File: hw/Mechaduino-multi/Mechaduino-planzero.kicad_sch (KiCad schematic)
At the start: 29 parts, among them IC1 A4954ELPTR-T, J2 SPI, J3 SPI_PWR, J4 Conn_01x04, J5 Conn_01x02, U1 ATtiny24-20MU, U2 AS5047D, U3 TLV70033_SOT353

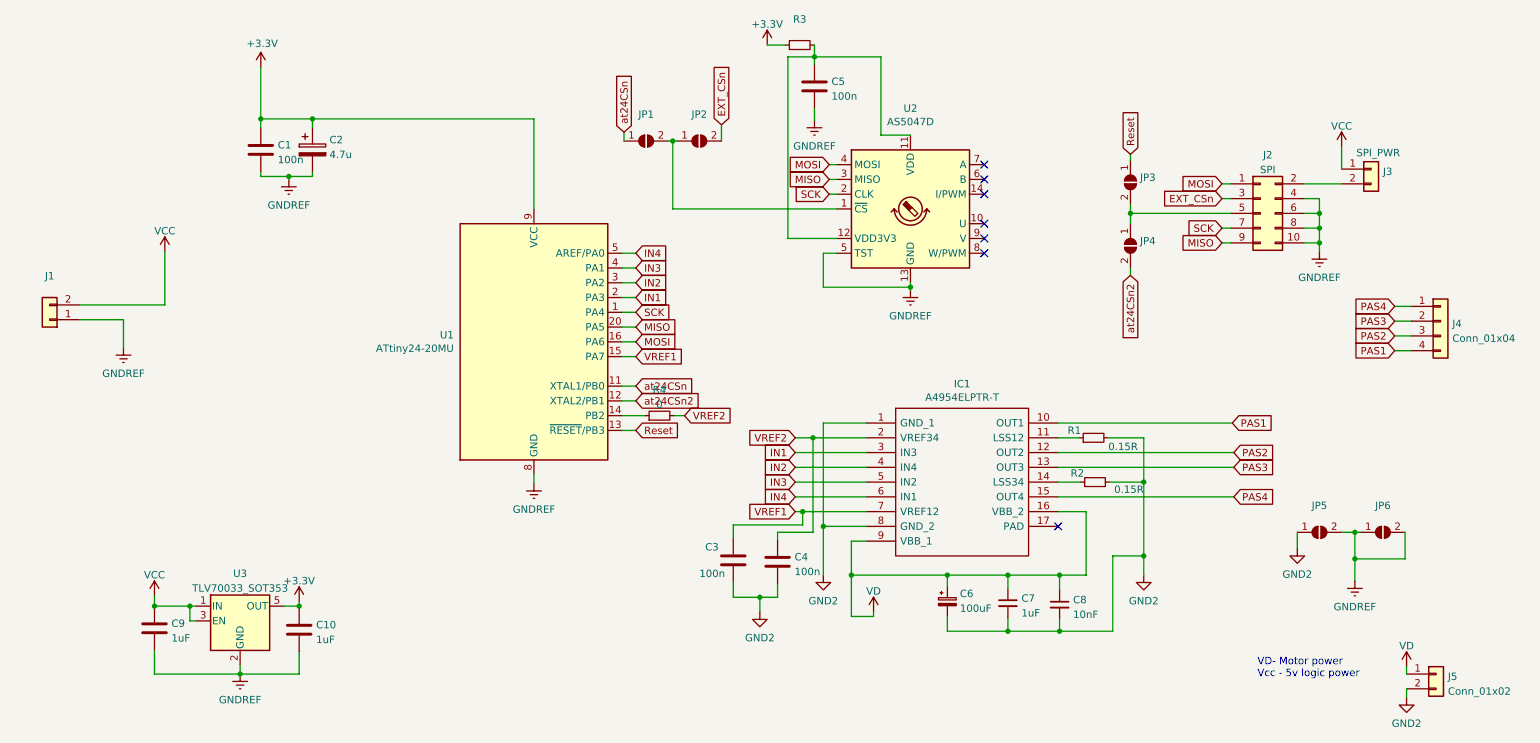
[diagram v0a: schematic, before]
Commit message: Add new updates to driver sch / layout
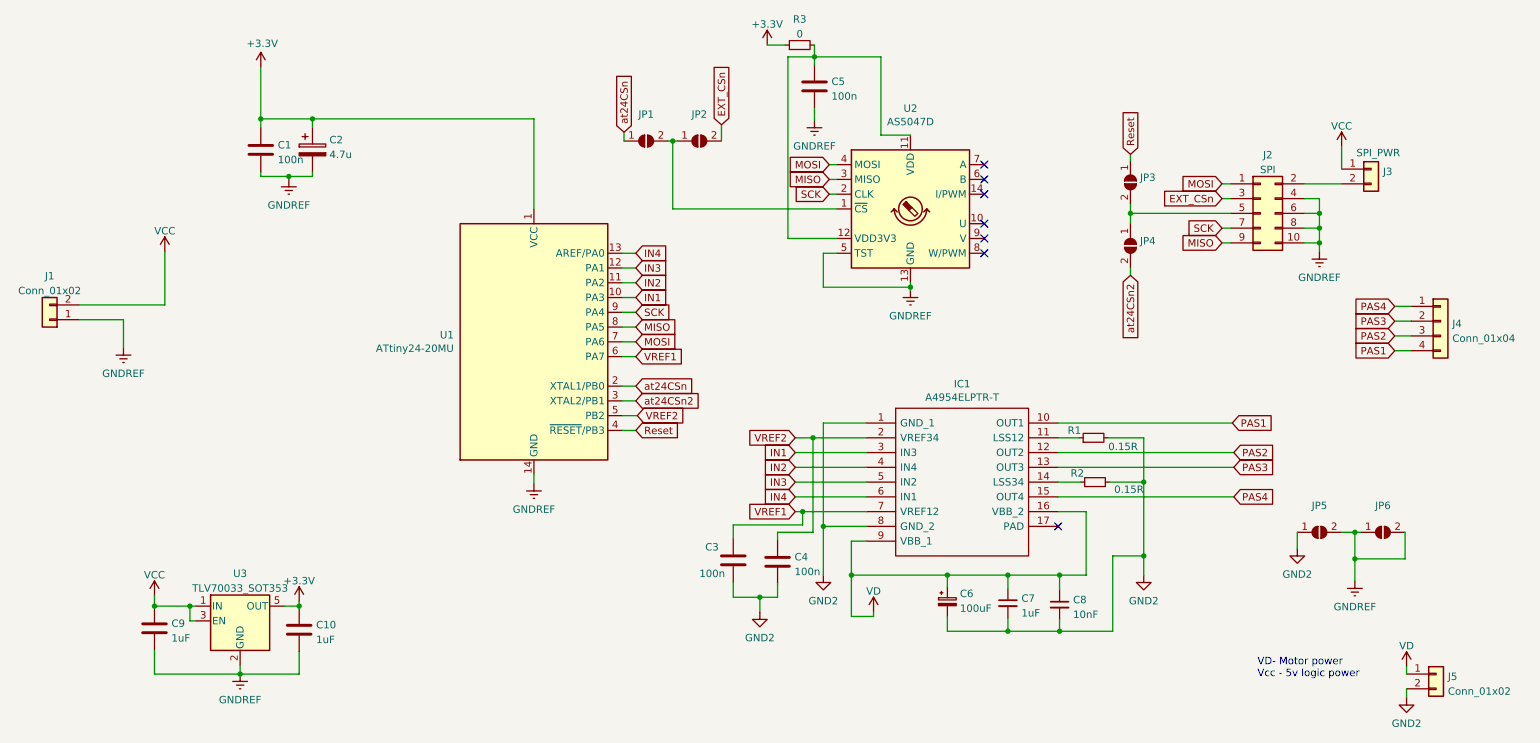
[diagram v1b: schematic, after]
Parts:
- removed R4: 0, Resistor_SMD:R_0805_2012Metric_Pad1.20x1.40mm_HandSolder, symbol Device:R_Small
- IC1: footprint (none) -> Package_SO:TSSOP-16-1EP_4.4x5mm_P0.65mm_EP3x3mm
- J1: value (none) -> Conn_01x02; footprint (none) -> Connector_PinSocket_2.54mm:PinSocket_1x02_P2.54mm_Horizontal
- J3: footprint (none) -> Connector_PinSocket_2.54mm:PinSocket_1x02_P2.54mm_Vertical
- R3: value (none) -> 0; footprint (none) -> Resistor_SMD:R_0805_2012Metric_Pad1.20x1.40mm_HandSolder
- U1: footprint Package_DFN_QFN:QFN-20-1EP_4x4mm_P0.5mm_EP2.6x2.6mm -> Package_SO:SOIC-14_3.9x8.7mm_P1.27mm; symbol Mechaduino-planzero-rescue:ATtiny24-20MU-MCU_Microchip_ATtiny -> MCU_Microchip_ATtiny:ATtiny24-20SSU
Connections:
- net +3V3: now also U1.1 (VCC); no longer U1.9 (VCC)
- net GNDREF: now also U1.14 (GND); no longer U1.21 (GND), U1.8 (GND)
- net IN1: now also U1.10 (PA3); no longer U1.2 (PA3)
- net IN2: now also U1.11 (PA2); no longer U1.3 (PA2)
- net IN3: now also U1.12 (PA1); no longer U1.4 (PA1)
- net IN4: now also U1.13 (AREF/PA0); no longer U1.5 (AREF/PA0)
- net MISO: now also U1.8 (PA5); no longer U1.20 (PA5)
- net MOSI: now also U1.7 (PA6); no longer U1.16 (PA6)
- net Reset: now also U1.4 (~{RESET}/PB3); no longer U1.13 (~{RESET}/PB3)
- net SCK: now also U1.9 (PA4); no longer U1.1 (PA4)
- net VREF1: now also U1.6 (PA7); no longer U1.15 (PA7)
- net VREF2: now also U1.5 (PB2)
- net at24CSn: now also U1.2 (XTAL1/PB0); no longer U1.11 (XTAL1/PB0)
- net at24CSn2: now also U1.3 (XTAL2/PB1); no longer U1.12 (XTAL2/PB1)
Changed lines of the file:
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@@
-    (stroke (width 0) (type default) (color 0 0 0 0))
-  )
-  (wire (pts (xy 137.16 81.28) (xy 138.938 81.28))
     (stroke (width 0) (type default) (color 0 0 0 0))
   )
@@
     (stroke (width 0) (type default) (color 0 0 0 0))
   )
-  (wire (pts (xy 128.27 81.28) (xy 132.08 81.28))
+  (wire (pts (xy 128.27 81.28) (xy 130.81 81.28))
     (stroke (width 0) (type default) (color 0 0 0 0))
   )
@@
     )
   )
-  (global_label "VREF2" (shape input) (at 138.938 81.28 0) (fields_autoplaced)
-    (effects (font (size 1.27 1.27)) (justify left))
-    (property "Intersheet References" "${INTERSHEET_REFS}" (id 0) (at 147.0679 81.2006 0)
+  (global_label "VREF2" (shape input) (at 130.81 81.28 0) (fields_autoplaced)
+    (effects (font (size 1.27 1.27)) (justify left))
+    (property "Intersheet References" "${INTERSHEET_REFS}" (id 0) (at 138.9399 81.2006 0)
       (effects (font (size 1.27 1.27)) (justify left) hide)
     )
@@
     (property "Reference" "IC1" (id 0) (at 186.69 75.819 0))
     (property "Value" "A4954ELPTR-T" (id 1) (at 186.69 78.1304 0))
-    (property "Footprint" "" (id 2) (at 199.39 80.01 0)
+    (property "Footprint" "Package_SO:TSSOP-16-1EP_4.4x5mm_P0.65mm_EP3x3mm" (id 2) (at 199.39 80.01 0)
       (effects (font (size 1.27 1.27)) (justify left) hide)
     )
@@
     (pin "9")
   )
-  (symbol (lib_id "Mechaduino-planzero-rescue:ATtiny24-20MU-MCU_Microchip_ATtiny") (at 113.03 68.58 0) (unit 1)
+  (symbol (lib_id "MCU_Microchip_ATtiny:ATtiny24-20SSU") (at 113.03 68.58 0) (unit 1)
     (in_bom yes) (on_board yes)
     (property "Reference" "U1" (id 0) (at 99.2378 67.4116 0)
@@
       (effects (font (size 1.27 1.27)) (justify right))
     )
-    (property "Footprint" "Package_DFN_QFN:QFN-20-1EP_4x4mm_P0.5mm_EP2.6x2.6mm" (id 2) (at 113.03 68.58 0)
+    (property "Footprint" "Package_SO:SOIC-14_3.9x8.7mm_P1.27mm" (id 2) (at 113.03 68.58 0)
       (effects (font (size 1.27 1.27) italic) hide)
     )
@@
     (pin "13")
     (pin "14")
-    (pin "15")
-    (pin "16")
-    (pin "17")
-    (pin "18")
-    (pin "19")
-    (pin "2")
-    (pin "20")
-    (pin "21")
+    (pin "2")
     (pin "3")
     (pin "4")
@@
     (in_bom yes) (on_board yes) (fields_autoplaced)
     (property "Reference" "R3" (id 0) (at 158.75 13.0896 90))
-    (property "Value" "" (id 1) (at 158.75 15.6265 90))
-    (property "Footprint" "" (id 2) (at 158.75 17.526 0)
+    (property "Value" "0" (id 1) (at 158.75 15.6265 90))
+    (property "Footprint" "Resistor_SMD:R_0805_2012Metric_Pad1.20x1.40mm_HandSolder" (id 2) (at 158.75 17.526 0)
       (effects (font (size 1.27 1.27)) hide)
     )
@@
       (effects (font (size 1.27 1.27)) (justify left))
     )
-    (property "Footprint" "" (id 2) (at 257.048 38.862 0)
+    (property "Footprint" "Connector_PinSocket_2.54mm:PinSocket_1x02_P2.54mm_Vertical" (id 2) (at 257.048 38.862 0)
       (effects (font (size 1.27 1.27)) hide)
     )
@@
     (pin "1")
   )
-  (symbol (lib_id "Device:R_Small") (at 134.62 81.28 90) (unit 1)
-    (in_bom yes) (on_board yes) (fields_autoplaced)
-    (property "Reference" "R4" (id 0) (at 134.62 76.8436 90))
-    (property "Value" "0" (id 1) (at 134.62 79.3805 90))
-    (property "Footprint" "Resistor_SMD:R_0805_2012Metric_Pad1.20x1.40mm_HandSolder" (id 2) (at 134.62 81.28 0)
-      (effects (font (size 1.27 1.27)) hide)
-    )
-    (property "Datasheet" "~" (id 3) (at 134.62 81.28 0)
-      (effects (font (size 1.27 1.27)) hide)
-    )
-    (pin "1")
-    (pin "2")
-  )
   (symbol (lib_id "power:GND2") (at 263.144 129.794 0) (unit 1)
     (in_bom yes) (on_board yes) (fields_autoplaced)
@@
     (in_bom yes) (on_board yes) (fields_autoplaced)
     (property "Reference" "J1" (id 0) (at 29.718 57.2602 0))
-    (property "Value" "" (id 1) (at 29.718 59.7971 0))
-    (property "Footprint" "" (id 2) (at 29.718 64.77 0)
+    (property "Value" "Conn_01x02" (id 1) (at 29.718 59.7971 0))
+    (property "Footprint" "Connector_PinSocket_2.54mm:PinSocket_1x02_P2.54mm_Horizontal" (id 2) (at 29.718 64.77 0)
       (effects (font (size 1.27 1.27)) hide)
     )
@@
       (reference "R3") (unit 1) (value "0") (footprint "Resistor_SMD:R_0805_2012Metric_Pad1.20x1.40mm_HandSolder")
     )
-    (path "/d22da0f2-72ba-4aff-bbb1-61dd4e95a1ce"
-      (reference "R4") (unit 1) (value "0") (footprint "Resistor_SMD:R_0805_2012Metric_Pad1.20x1.40mm_HandSolder")
-    )
     (path "/00000000-0000-0000-0000-0000634c0410"
-      (reference "U1") (unit 1) (value "ATtiny24-20MU") (footprint "Package_DFN_QFN:QFN-20-1EP_4x4mm_P0.5mm_EP2.6x2.6mm")
+      (reference "U1") (unit 1) (value "ATtiny24-20MU") (footprint "Package_SO:SOIC-14_3.9x8.7mm_P1.27mm")
     )
     (path "/00000000-0000-0000-0000-0000634c169e"
